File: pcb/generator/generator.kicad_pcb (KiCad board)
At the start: 2 copper layers, 77.5 x 104.5 mm, 53 parts, among them J1 Power, J2 SWD, J3 CH1, J4 CH2, J5 USB, U1 ATSAMD11D14A-SS, U2 SRH05S3V3, U3 L6206D, U4 MCP9700T-HLT, U5 LP2985-3.3, U6 SN65220, Y1 32.768kHz

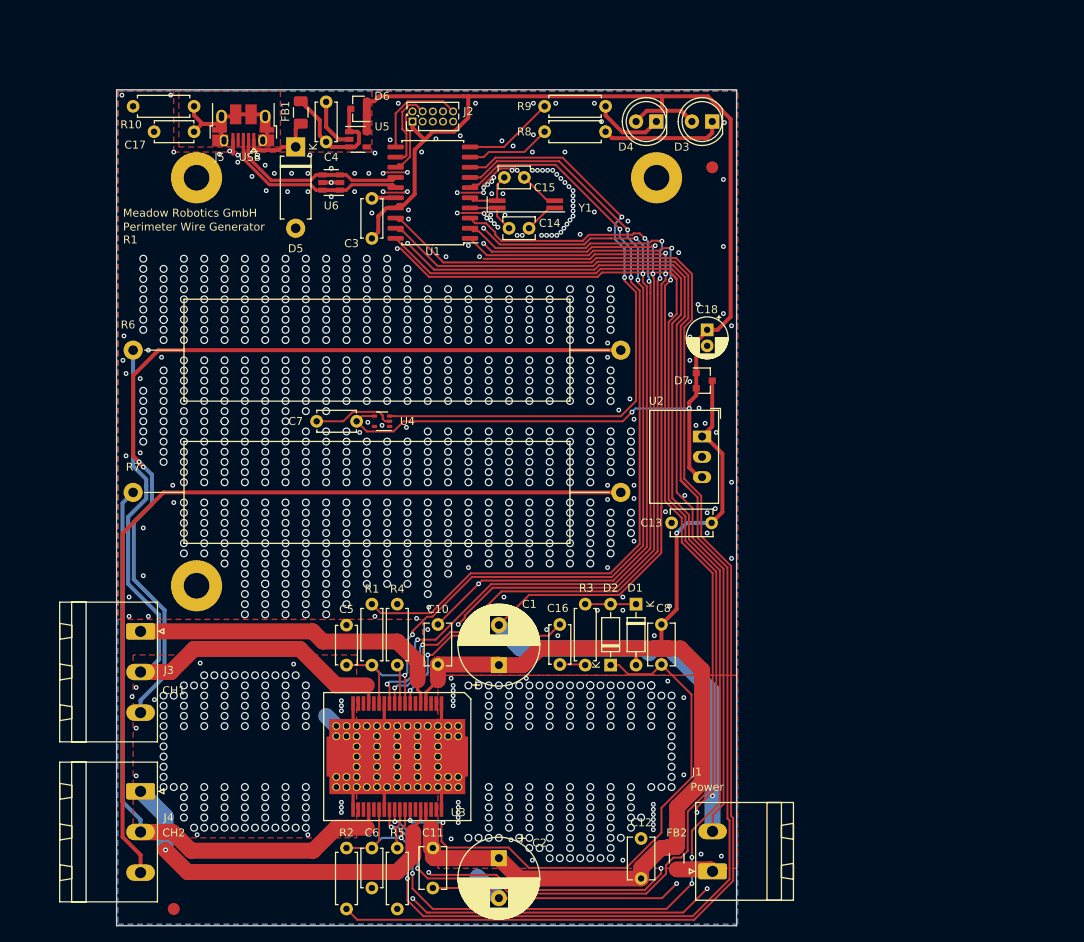
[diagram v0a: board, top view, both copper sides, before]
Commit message: generator: pcb for modulbox
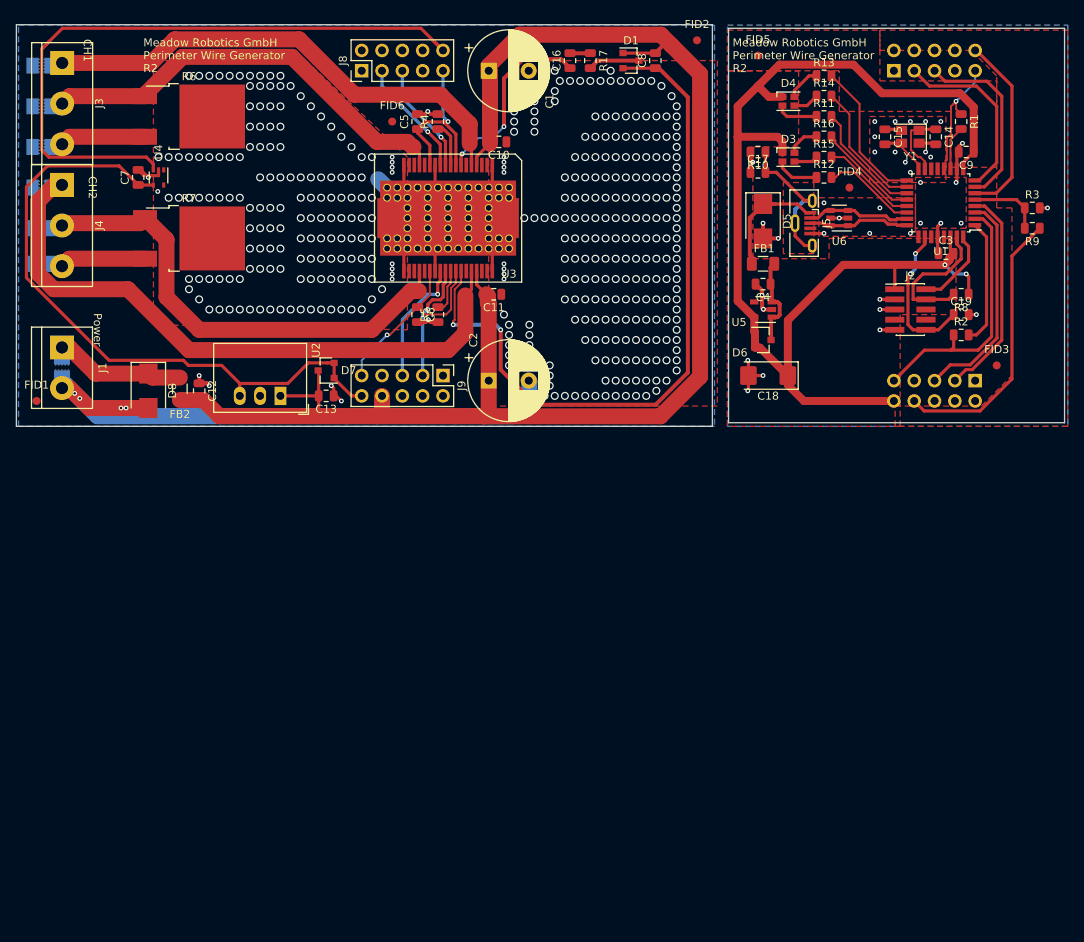
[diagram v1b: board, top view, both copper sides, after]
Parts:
- removed D2: D, Diode_THT:D_DO-35_SOD27_P7.62mm_Horizontal
- removed H1, H2, H3: MountingHole_Pad, MountingHole:MountingHole_3.2mm_M3_Pad
- added C19: 100n, Capacitor_SMD:C_0805_2012Metric, F.Cu at (155.6, 78.1)
- added C9: 100n, Capacitor_SMD:C_0805_2012Metric, F.Cu at (156.2, 57.8)
- added D8: 48V, Diode_SMD:D_SMB, F.Cu at (54.0, 87.6)
- added E1: SPARK_GAP, footprints:Spark_Gap_0.4_Pwr, B.Cu at (43.2, 84.7)
- added E2: SPARK_GAP, footprints:Spark_Gap_0.4_Pwr, B.Cu at (40.6, 47.0)
- added E3: SPARK_GAP, footprints:Spark_Gap_0.4_Pwr, B.Cu at (40.6, 52.1)
- added E4: SPARK_GAP, footprints:Spark_Gap_0.4_Pwr, B.Cu at (40.6, 57.1)
- added E5: SPARK_GAP, footprints:Spark_Gap_0.4_Pwr, B.Cu at (40.6, 62.2)
- added E6: SPARK_GAP, footprints:Spark_Gap_0.4_Pwr, B.Cu at (40.6, 67.3)
- added E7: SPARK_GAP, footprints:Spark_Gap_0.4_Pwr, B.Cu at (40.6, 71.8)
- added FID3: Fiducial, Fiducial:Fiducial_1mm_Mask2mm, F.Cu at (160.0, 84.5)
- added FID4: Fiducial, Fiducial:Fiducial_1mm_Mask2mm, F.Cu at (141.6, 62.2)
- added FID5: Fiducial, Fiducial:Fiducial_1mm_Mask2mm, F.Cu at (130.2, 45.7)
- added FID6: Fiducial, Fiducial:Fiducial_1mm_Mask2mm, F.Cu at (84.5, 54.0)
- added J6: Au, Connector_PinSocket_2.54mm:PinSocket_2x05_P2.54mm_Vertical, B.Cu at (147.2, 47.6)
- added J7: Bu, Connector_PinSocket_2.54mm:PinSocket_2x05_P2.54mm_Vertical, B.Cu at (157.3, 86.4)
- added J8: Al, Connector_PinHeader_2.54mm:PinHeader_2x05_P2.54mm_Vertical, F.Cu at (80.6, 47.6)
- added J9: Bl, Connector_PinHeader_2.54mm:PinHeader_2x05_P2.54mm_Vertical, F.Cu at (90.8, 85.7)
- added R11: 280R, Resistor_SMD:R_0805_2012Metric, F.Cu at (138.4, 53.3)
- added R12: 280R, Resistor_SMD:R_0805_2012Metric, F.Cu at (138.4, 61.0)
- added R13: 100R, Resistor_SMD:R_0805_2012Metric, F.Cu at (138.4, 48.3)
- added R14: 100R, Resistor_SMD:R_0805_2012Metric, F.Cu at (138.4, 50.8)
- added R15: 100R, Resistor_SMD:R_0805_2012Metric, F.Cu at (138.4, 58.4)
- added R16: 100R, Resistor_SMD:R_0805_2012Metric, F.Cu at (138.4, 55.9)
- added R17: 100R, Resistor_SMD:R_0805_2012Metric, F.Cu at (109.2, 46.4)
- C10, C11, C12, C13, C8: footprint Capacitor_THT:C_Disc_D5.1mm_W3.2mm_P5.00mm -> Capacitor_SMD:C_0805_2012Metric
- C14, C15: value 20p -> 22p; footprint Capacitor_THT:C_Disc_D3.8mm_W2.6mm_P2.50mm -> Capacitor_SMD:C_0805_2012Metric
- C16, C17, C3, C4, C5, C6, C7: footprint Capacitor_THT:C_Disc_D4.7mm_W2.5mm_P5.00mm -> Capacitor_SMD:C_0805_2012Metric
- C18: footprint Capacitor_THT:CP_Radial_D5.0mm_P2.00mm -> Capacitor_Tantalum_SMD:CP_EIA-6032-28_Kemet-C
- D1: footprint Diode_THT:D_DO-35_SOD27_P7.62mm_Horizontal -> Package_TO_SOT_SMD:SOT-23
- D3: value Red1 -> CLMVC-FKA; footprint LED_THT:LED_D5.0mm -> LED_SMD:LED_Cree-PLCC4_2x2mm_CW
- D4: value Red2 -> CLMVC-FKA; footprint LED_THT:LED_D5.0mm -> LED_SMD:LED_Cree-PLCC4_2x2mm_CW
- D5: footprint Diode_THT:D_DO-15_P10.16mm_Horizontal -> Diode_SMD:D_SMB
- FB1: value BLM31KN471SN1L -> BLM31KN471SN1L
- FB2: value BLM31SN500SN1 -> BLM31SN500SN1L
- FID1, FID2: footprint Fiducial:Fiducial_1.5mm_Mask3mm -> Fiducial:Fiducial_1mm_Mask2mm
- J1: footprint Connector_Phoenix_MSTB:PhoenixContact_MSTBA_2,5_2-G_1x02_P5.00mm_Horizontal -> TerminalBlock:TerminalBlock_bornier-2_P5.08mm
- J2: footprint Connector_PinHeader_1.27mm:PinHeader_2x05_P1.27mm_Vertical -> Connector_PinHeader_1.27mm:PinHeader_2x05_P1.27mm_Vertical_SMD
- J3, J4: footprint Connector_Phoenix_MSTB:PhoenixContact_MSTBA_2,5_3-G-5,08_1x03_P5.08mm_Horizontal -> TerminalBlock:TerminalBlock_bornier-3_P5.08mm
- J5: footprint Connector_USB:USB_Micro-B_Amphenol_10103594-0001LF_Horizontal -> Connector_USB:USB_Micro-B_Molex-105133-0001
- R1, R2: value 10k -> 22k; footprint Resistor_THT:R_Axial_DIN0207_L6.3mm_D2.5mm_P7.62mm_Horizontal -> Resistor_SMD:R_0805_2012Metric
- R10, R4, R5: footprint Resistor_THT:R_Axial_DIN0207_L6.3mm_D2.5mm_P7.62mm_Horizontal -> Resistor_SMD:R_0805_2012Metric
- R3: value 100 -> 22k; footprint Resistor_THT:R_Axial_DIN0207_L6.3mm_D2.5mm_P7.62mm_Horizontal -> Resistor_SMD:R_0805_2012Metric
- R6, R7: value 240 -> 200R; footprint Resistor_THT:R_Axial_Power_L48.0mm_W12.5mm_P60.96mm -> footprints:Ohmite-TKH
- R8: value 750R -> 1k; footprint Resistor_THT:R_Axial_DIN0207_L6.3mm_D2.5mm_P7.62mm_Horizontal -> Resistor_SMD:R_0805_2012Metric
- R9: value 750R -> 1M; footprint Resistor_THT:R_Axial_DIN0207_L6.3mm_D2.5mm_P7.62mm_Horizontal -> Resistor_SMD:R_0805_2012Metric
- U1: value ATSAMD11D14A-SS -> ATSAMD21E; footprint Package_SO:SOIC-20W_7.5x12.8mm_P1.27mm -> Package_QFP:TQFP-32_7x7mm_P0.8mm
- U3: value L6206D -> L6206
- Y1: value 32.768kHz -> 16MHz; footprint Crystal:Crystal_SMD_SeikoEpson_MC146-4Pin_6.7x1.5mm_HandSoldering -> Crystal:Crystal_SMD_SeikoEpson_TSX3225-4Pin_3.2x2.5mm
- moved J1 104.4 mm to (43.2, 82.2), turned to 270 degrees
- moved R1 100.2 mm to (155.6, 54.0), turned to 270 degrees
- moved R2 100.1 mm to (155.6, 80.6), turned to 0 degrees
- moved FB2 85.4 mm to (57.9, 87.4), turned to 90 degrees
- moved R3 79.9 mm to (164.5, 64.8), turned to 0 degrees
- moved C12 78.6 mm to (60.3, 87.6)
- moved J4 76.4 mm to (43.2, 61.9)
- moved C17 75.7 mm to (130.2, 60.3)
- moved C8 75.5 mm to (117.3, 46.4)
- moved C11 74.6 mm to (97.2, 75.6), turned to 180 degrees
- moved R5 74.5 mm to (90.2, 78.1)
- moved C1 74.3 mm to (96.5, 47.6), turned to 0 degrees
- moved C3 72.1 mm to (153.7, 70.5), turned to 0 degrees
- moved J3 71.7 mm to (43.2, 46.6)
- moved J5 71.1 mm to (135.9, 66.7), turned to 270 degrees
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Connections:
- D1 pad 1: Net-(D1-Pad1) -> +48V
- D1 pad 2: +48V -> Net-(C8-Pad1)
- D3 pad 1: Net-(D3-Pad1) -> +3V3
- D3 pad 2: +3V3 -> Net-(D3-Pad2)
- D4 pad 1: Net-(D4-Pad1) -> +3V3
- D4 pad 2: +3V3 -> Net-(D4-Pad2)
- J3 pad 2: Net-(J3-Pad2) -> Net-(E3-Pad1)
- J3 pad 3: Net-(J3-Pad3) -> Net-(E4-Pad1)
- J4 pad 2: Net-(J4-Pad2) -> Net-(E6-Pad1)
- J4 pad 3: Net-(J4-Pad3) -> Net-(E7-Pad1)
- R3 pad 1: Net-(C16-Pad2) -> /V_SENSE
- R3 pad 2: Net-(D1-Pad1) -> GND
- R6 pad 1: Net-(J3-Pad3) -> Net-(E3-Pad1)
- R6 pad 2: Net-(J3-Pad2) -> GND
- R7 pad 1: Net-(J4-Pad3) -> Net-(E6-Pad1)
- R7 pad 2: Net-(J4-Pad2) -> GND
- R8 pad 1: Net-(D3-Pad1) -> +3V3
- R8 pad 2: Net-(R8-Pad2) -> /SWCLK
- R9 pad 1: Net-(D4-Pad1) -> +48V
- R9 pad 2: Net-(R9-Pad2) -> /V_SENSE
- U1 pad 1: /IN2_B -> /EN_B
- U1 pad 10: Net-(R9-Pad2) -> GND
- U1 pad 11: /~RESET -> /EN_A
- U1 pad 12: /SWCLK -> /ERROR_A
- U1 pad 13: /SWDIO -> (no net)
- U1 pad 14: /USB_D- -> (no net)
- U1 pad 15: /USB_D+ -> Net-(C14-Pad1)
- U1 pad 16: GND -> Net-(C15-Pad2)
- U1 pad 17: +3V3 -> Net-(R13-Pad2)
- U1 pad 18: /EN_B -> Net-(R14-Pad2)
- U1 pad 19: /ERROR_B -> Net-(R11-Pad2)
- U1 pad 2: /IN1_A -> /ERROR_B
- U1 pad 20: /IN1_B -> Net-(R16-Pad2)
- U1 pad 3: /IN2_A -> /IN1_B
- U1 pad 4: Net-(C14-Pad1) -> /IN2_B
- U1 pad 5: Net-(C15-Pad2) -> /V_SENSE
- U1 pad 6: /EN_A -> /R_TEMP
- U1 pad 7: /ERROR_A -> /IN1_A
- U1 pad 8: /R_TEMP -> /IN2_A
- U1 pad 9: Net-(R8-Pad2) -> +3V3
- U3 pad 15: Net-(J3-Pad2) -> Net-(E3-Pad1)
- U3 pad 22: Net-(J4-Pad2) -> Net-(E6-Pad1)
- Y1 pad 3: GND -> Net-(C15-Pad2)
- Y1 pad 4: Net-(C15-Pad2) -> GND
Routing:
- net GND: track 641.8 -> 162.0 mm, vias 1102 -> 434
- net /EN_B: track 170.1 -> 15.8 mm
- net /ERROR_B: track 186.5 -> 59.4 mm, vias 2 -> 1
- net /IN1_B: track 167.1 -> 43.3 mm, vias 4 -> 1
- net /IN2_B: track 152.7 -> 41.7 mm, vias 4 -> 1
- net Net-(J3-Pad3): track 110.0 -> 0.00 mm, vias 2 -> 0
- net Net-(J4-Pad3): track 108.4 -> 0.00 mm
- net /EN_A: track 101.1 -> 5.53 mm, vias 2 -> 0
- net /ERROR_A: track 120.1 -> 37.8 mm, vias 4 -> 2
- net Net-(J4-Pad2): track 80.6 -> 0.00 mm
- net Net-(J3-Pad2): track 78.6 -> 0.00 mm
- net /IN1_A: track 108.2 -> 37.2 mm, vias 4 -> 1
- net +48V: track 151.8 -> 222.7 mm, vias 1 -> 0
- net (no net): track 70.3 -> 0.00 mm, vias 4 -> 0
- net /IN2_A: track 107.6 -> 37.7 mm, vias 4 -> 1
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- added copper zone on F.Cu, net +3V3
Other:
- board size 77.5 x 104.5 mm -> 131 x 50.2 mm
- net class Default: clearance 0.2 -> 0.19
- rule trace_clearance: 0.2 -> 0.19
- board text added: "Meadow Robotics GmbH Perimeter Wire Generator R2"
- board text removed: "Meadow Robotics GmbH"
- board text removed: "Perimeter Wire Generator R1"
- board text removed: "USB"
